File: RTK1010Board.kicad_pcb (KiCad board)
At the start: 2 copper layers, 56.2 x 53.3 mm, 75 parts, among them J1 SMA, J2 IPEX, J3 USB_OTG, J4 BNO055, U1 RTK-1010, U2 NCP1117-3.3_SOT223, U3 MCP1700-3302E_SOT23, U4 ESP32-S2-WROVER

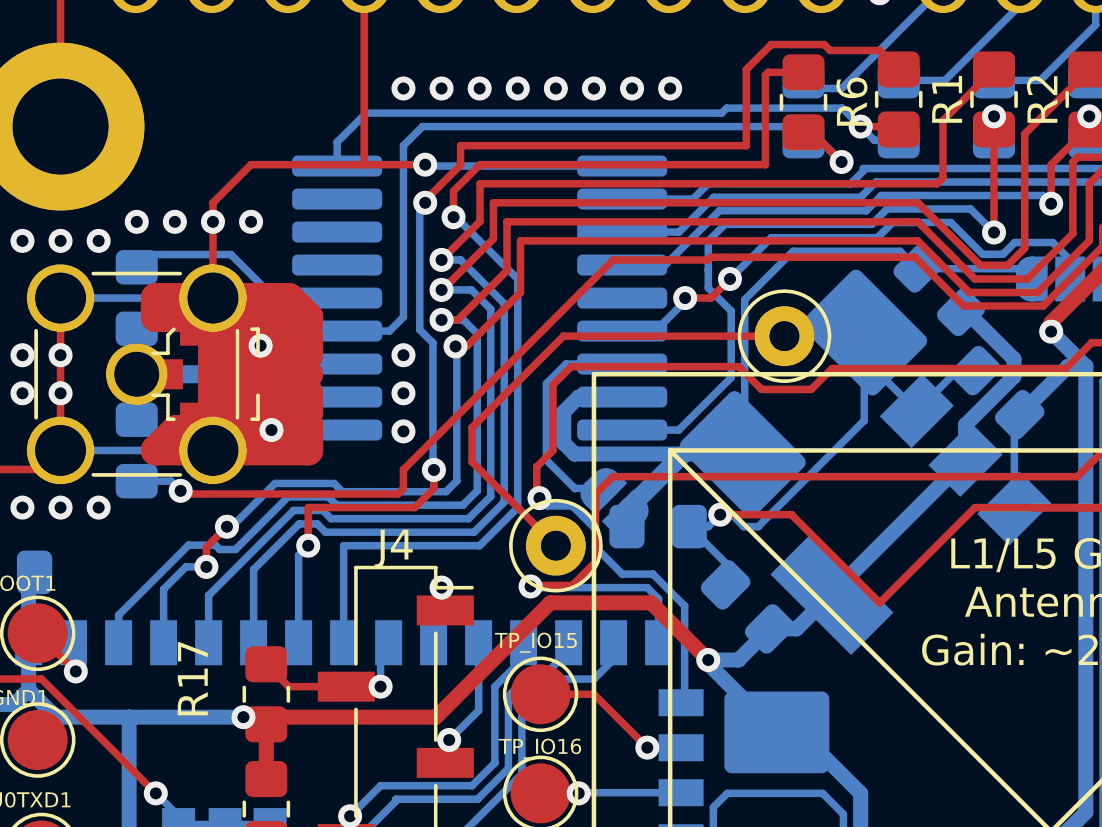
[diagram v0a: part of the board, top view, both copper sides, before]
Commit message: ibom added
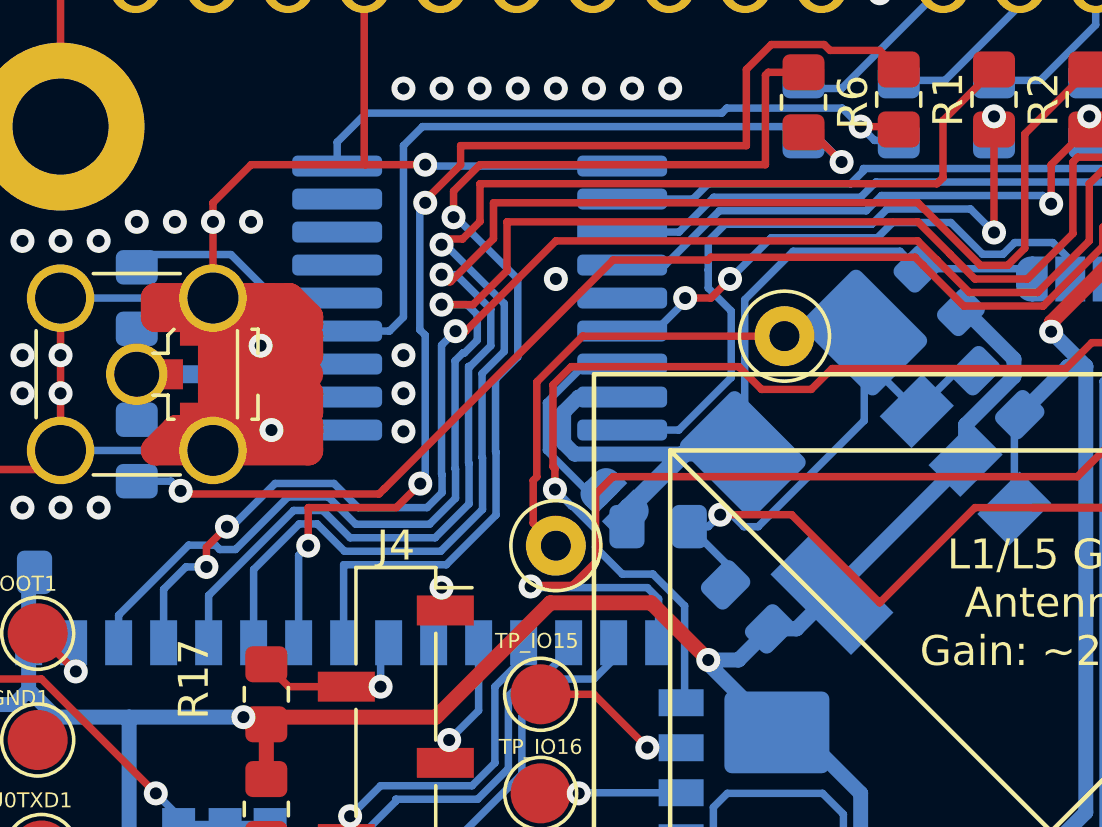
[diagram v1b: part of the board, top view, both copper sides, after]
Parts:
- L3: value ?H -> 1.2uH
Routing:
- net GND: track 425.5 -> 423.4 mm, vias 67 -> 68
- net Net-(R20-Pad1): track 38.4 -> 37.5 mm
- net Net-(R5-Pad1): track 54.0 -> 54.6 mm
- net Net-(R6-Pad1): track 36.1 -> 35.5 mm
- net Net-(R1-Pad1): track 39.1 -> 38.5 mm
- net Net-(JP3-Pad2): track 7.55 -> 6.98 mm

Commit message: ibom updated
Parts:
- C2, C3: value 100nF -> 100pF
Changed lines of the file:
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@@
     (property "Sheetfile" "RTK1010Board.kicad_sch")
     (property "Sheetname" "")
-    (property "Variant" "B")
+    (property "Variant" "VarB")
     (attr smd)
     (fp_text reference "C12" (at -6.35 1.905) (layer "F.SilkS")
@@
     (property "Sheetfile" "RTK1010Board.kicad_sch")
     (property "Sheetname" "")
-    (property "Variant" "A,B")
+    (property "Variant" "VarA,VarB")
     (attr smd)
     (fp_text reference "J2" (at 5.08 1.905) (layer "F.SilkS") hide
@@
     (property "Sheetfile" "RTK1010Board.kicad_sch")
     (property "Sheetname" "")
-    (property "Variant" "B")
+    (property "Variant" "VarB")
     (attr smd)
     (fp_text reference "R5" (at 0 -1.65 90) (layer "F.SilkS")
@@
     (property "Sheetfile" "RTK1010Board.kicad_sch")
     (property "Sheetname" "")
-    (property "Variant" "A")
+    (property "Variant" "VarA")
     (attr through_hole)
     (fp_text reference "XA1" (at 7.62 -54.61) (layer "F.SilkS") hide
@@
     (property "Sheetfile" "RTK1010Board.kicad_sch")
     (property "Sheetname" "")
-    (property "Variant" "B")
+    (property "Variant" "VarB")
     (attr smd)
     (fp_text reference "R4" (at 0 -1.65 90) (layer "F.SilkS")
@@
     (property "Sheetfile" "RTK1010Board.kicad_sch")
     (property "Sheetname" "")
+    (property "Variant" "VarB")
     (attr smd)
     (fp_text reference "U4" (at 2.62 2.235 180) (layer "B.SilkS")
@@
     (property "Sheetfile" "RTK1010Board.kicad_sch")
     (property "Sheetname" "")
-    (property "Variant" "")
+    (property "Variant" "VarB")
     (attr smd)
     (fp_text reference "C3" (at -3.02795 0.011857 135) (layer "B.SilkS")
       (effects (font (size 1 1) (thickness 0.15)) (justify mirror))
     )
-    (fp_text value "100nF" (at 0 -1.68 135) (layer "B.Fab")
+    (fp_text value "100pF" (at 0 -1.68 135) (layer "B.Fab")
       (effects (font (size 1 1) (thickness 0.15)) (justify mirror))
     )
@@
     (property "Sheetfile" "RTK1010Board.kicad_sch")
     (property "Sheetname" "")
+    (property "Variant" "VarB")
     (attr smd)
     (fp_text reference "C11" (at 0 -0.254 135) (layer "B.SilkS")
@@
     (property "Sheetfile" "RTK1010Board.kicad_sch")
     (property "Sheetname" "")
-    (property "Variant" "A,B")
+    (property "Variant" "VarA,VarB")
     (attr smd)
     (fp_text reference "C5" (at 0 1.68) (layer "B.SilkS")
@@
     (property "Sheetfile" "RTK1010Board.kicad_sch")
     (property "Sheetname" "")
-    (property "Variant" "A")
+    (property "Variant" "VarA")
     (attr smd)
     (fp_text reference "R8" (at 2 1.27 180) (layer "B.SilkS")
@@
     (property "Sheetfile" "RTK1010Board.kicad_sch")
     (property "Sheetname" "")
-    (property "Variant" "B")
+    (property "Variant" "VarB")
     (attr smd)
     (fp_text reference "C2" (at -2.694077 0 135) (layer "B.SilkS")
       (effects (font (size 1 1) (thickness 0.15)) (justify mirror))
     )
-    (fp_text value "100nF" (at 0 -1.68 135) (layer "B.Fab")
+    (fp_text value "100pF" (at 0 -1.68 135) (layer "B.Fab")
       (effects (font (size 1 1) (thickness 0.15)) (justify mirror))
     )
@@
     (property "Sheetfile" "RTK1010Board.kicad_sch")
     (property "Sheetname" "")
-    (property "Variant" "A,B")
+    (property "Variant" "VarA,VarB")
     (attr smd)
     (fp_text reference "U1" (at 5.08 2.54 unlocked) (layer "B.Cu") hide
@@
     (property "Sheetfile" "RTK1010Board.kicad_sch")
     (property "Sheetname" "")
-    (property "Variant" "B")
+    (property "Variant" "VarB")
     (attr smd)
     (fp_text reference "R13" (at 0.449013 -4.041115 135) (layer "B.SilkS")
@@
     (property "Sheetfile" "RTK1010Board.kicad_sch")
     (property "Sheetname" "")
-    (property "Variant" "B")
+    (property "Variant" "VarB")
     (attr smd)
     (fp_text reference "R15" (at 2.81 -0.381) (layer "B.SilkS")
@@
     (property "Sheetfile" "RTK1010Board.kicad_sch")
     (property "Sheetname" "")
+    (property "Variant" "VarB")
     (attr smd)
     (fp_text reference "C4" (at 0 1.68 135) (layer "B.SilkS")
@@
     (property "Sheetfile" "RTK1010Board.kicad_sch")
     (property "Sheetname" "")
-    (property "Variant" "B")
+    (property "Variant" "VarB")
     (attr smd)
     (fp_text reference "C8" (at 0 1.68) (layer "B.SilkS")
@@
     (property "Sheetfile" "RTK1010Board.kicad_sch")
     (property "Sheetname" "")
+    (property "Variant" "VarB")
     (attr smd)
     (fp_text reference "C1" (at 0 1.68 135) (layer "B.SilkS")
@@
     (property "Sheetfile" "RTK1010Board.kicad_sch")
     (property "Sheetname" "")
-    (property "Variant" "A,B")
+    (property "Variant" "VarA,VarB")
     (attr smd)
     (fp_text reference "C13" (at 0 2.7 45) (layer "B.SilkS")
@@
     (property "Sheetfile" "RTK1010Board.kicad_sch")
     (property "Sheetname" "")
-    (property "Variant" "B")
+    (property "Variant" "VarB")
     (attr smd)
     (fp_text reference "C9" (at -0.2325 1.651 180) (layer "B.SilkS")
@@
     (property "Sheetfile" "RTK1010Board.kicad_sch")
     (property "Sheetname" "")
-    (property "Variant" "B")
+    (property "Variant" "VarB")
     (attr smd)
     (fp_text reference "R16" (at 1.143 -1.651) (layer "B.SilkS")
@@
     (property "Sheetfile" "RTK1010Board.kicad_sch")
     (property "Sheetname" "")
-    (property "Variant" "B")
+    (property "Variant" "VarB")
     (attr smd)
     (fp_text reference "R14" (at 0 1.65 135) (layer "B.SilkS")
@@
     (property "Sheetfile" "RTK1010Board.kicad_sch")
     (property "Sheetname" "")
-    (property "Variant" "A,B")
+    (property "Variant" "VarA,VarB")
     (attr smd)
     (fp_text reference "L1" (at -2.54 -0.635 90) (layer "B.SilkS")
@@
     (property "Sheetfile" "RTK1010Board.kicad_sch")
     (property "Sheetname" "")
-    (property "Variant" "B")
+    (property "Variant" "VarB")
     (attr smd)
     (fp_text reference "J3" (at -3.76 0.67) (layer "B.SilkS")
@@
     (property "Sheetfile" "RTK1010Board.kicad_sch")
     (property "Sheetname" "")
+    (property "Variant" "VarB")
     (attr smd)
     (fp_text reference "U2" (at 0 4.5 45) (layer "B.SilkS")
@@
     (property "Sheetfile" "RTK1010Board.kicad_sch")
     (property "Sheetname" "")
-    (property "Variant" "A")
+    (property "Variant" "VarA")
     (attr smd)
     (fp_text reference "R7" (at -2 -1.905 180) (layer "B.SilkS")

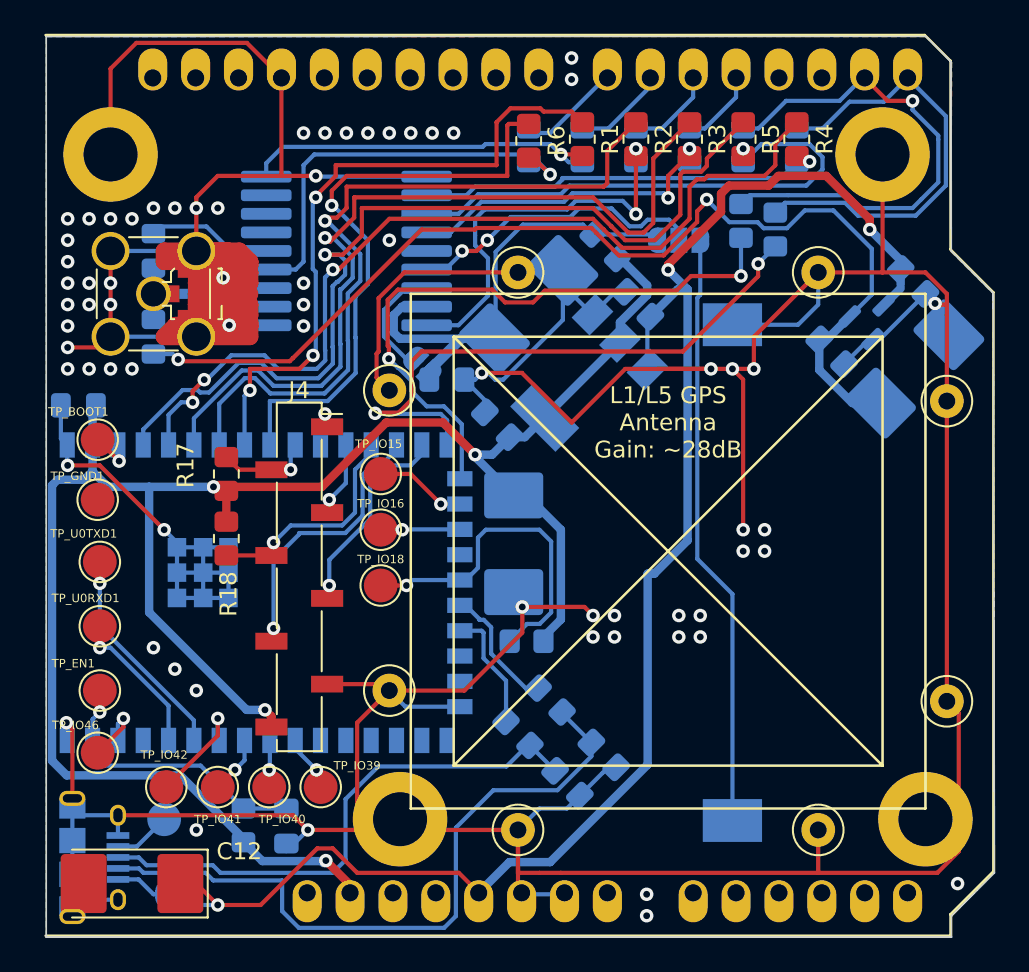
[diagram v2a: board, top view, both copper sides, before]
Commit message: V1.0
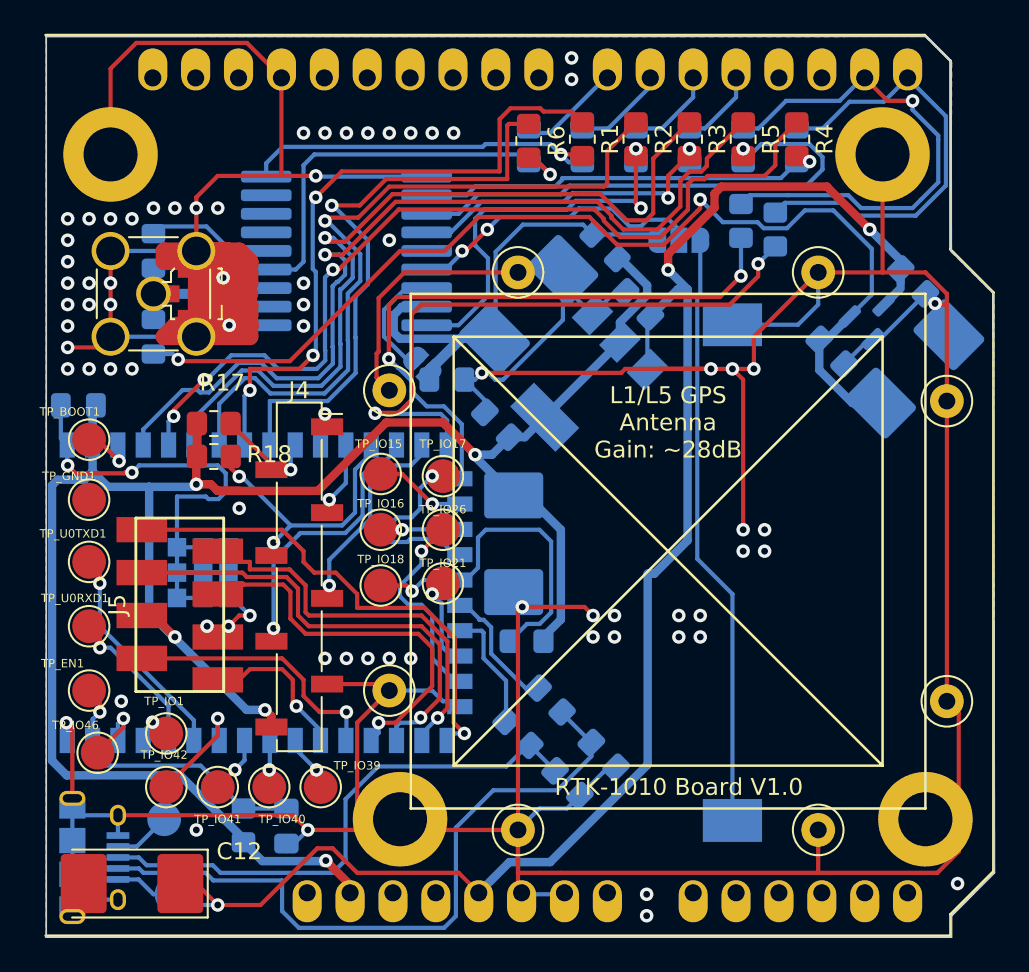
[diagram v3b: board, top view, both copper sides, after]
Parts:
- added J5: Conn_GPS, footprints:CONN-TE-MICROMATCH-4X2-SMD, F.Cu at (179.4, 107.3)
- added TP_IO1: TestPoint, TestPoint:TestPoint_Pad_D2.0mm, F.Cu at (178.6, 114.9)
- added TP_IO17: TestPoint, TestPoint:TestPoint_Pad_D2.0mm, F.Cu at (194.9, 99.7)
- added TP_IO21: TestPoint, TestPoint:TestPoint_Pad_D2.0mm, F.Cu at (194.9, 106.0)
- added TP_IO26: TestPoint, TestPoint:TestPoint_Pad_D2.0mm, F.Cu at (194.9, 102.9)
- moved R18 4.91 mm to (181.4, 98.5), turned to 0 degrees
- moved R17 3.08 mm to (181.4, 96.6), turned to 0 degrees
- moved TP_EN1 0.63 mm to (174.0, 112.4)
- moved TP_U0RXD1 0.63 mm to (174.0, 108.6)
- moved TP_U0TXD1 0.63 mm to (174.0, 104.8)
- moved TP_BOOT1 0.51 mm to (174.0, 97.5)
- moved TP_GND1 0.51 mm to (174.0, 101.1)
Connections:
- U4 pad 27: unconnected-(U4-Pad27) -> GPS_RXD
- U4 pad 28: unconnected-(U4-Pad28) -> GPS_SCL
- U4 pad 29: unconnected-(U4-Pad29) -> GPS_TXD
- U4 pad 30: unconnected-(U4-Pad30) -> GPS_SDA
- U4 pad 31: unconnected-(U4-Pad31) -> GPS_7
- U4 pad 32: unconnected-(U4-Pad32) -> GPS_8
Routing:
- net GPS_RXD: track 0.00 -> 29.2 mm, vias 0 -> 1
- net GPS_TXD: track 0.00 -> 27.8 mm, vias 0 -> 1
- net GPS_SCL: track 0.00 -> 23.5 mm, vias 0 -> 1
- net GPS_SDA: track 0.00 -> 23.1 mm, vias 0 -> 1
- net GPS_7: track 0.00 -> 15.7 mm, vias 0 -> 1
- net GND: track 423.4 -> 436.1 mm, vias 68 -> 75
- net unconnected-(U4-Pad25): track 0.00 -> 12.1 mm, vias 0 -> 1
- net unconnected-(U4-Pad20): track 0.00 -> 10.7 mm, vias 0 -> 1
- net GPS_8: track 0.00 -> 9.24 mm, vias 0 -> 1
- net +3V3: track 123.5 -> 130.6 mm, vias 4 -> 5
- net unconnected-(U4-Pad24): track 0.00 -> 5.54 mm, vias 0 -> 1
- net BNO_ADDR: track 13.4 -> 16.4 mm, vias 1 -> 2
- net unconnected-(U4-Pad39): track 0.00 -> 2.41 mm, vias 0 -> 1
- net Net-(R19-Pad1): track 35.5 -> 37.1 mm
- net Net-(R5-Pad1): track 54.6 -> 53.0 mm
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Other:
- board text added: "RTK-1010 Board V1.0"
